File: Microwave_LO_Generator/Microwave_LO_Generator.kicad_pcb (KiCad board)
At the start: 4 copper layers, 53.3 x 42.9 mm, 65 parts, among them J1 Conn_01x02_Male, J2 Conn_01x02_Male, J3 Conn_01x01_Female, J4 Conn_01x05_Male, J5 Conn_01x01_Female, U1 ADF4150HV, U2 LT1962-3.3, U3 LT3010, U4 SMT_24_ADI, U5 LT1962-5, U6 LT1962-5, X1 IQXT-220-1

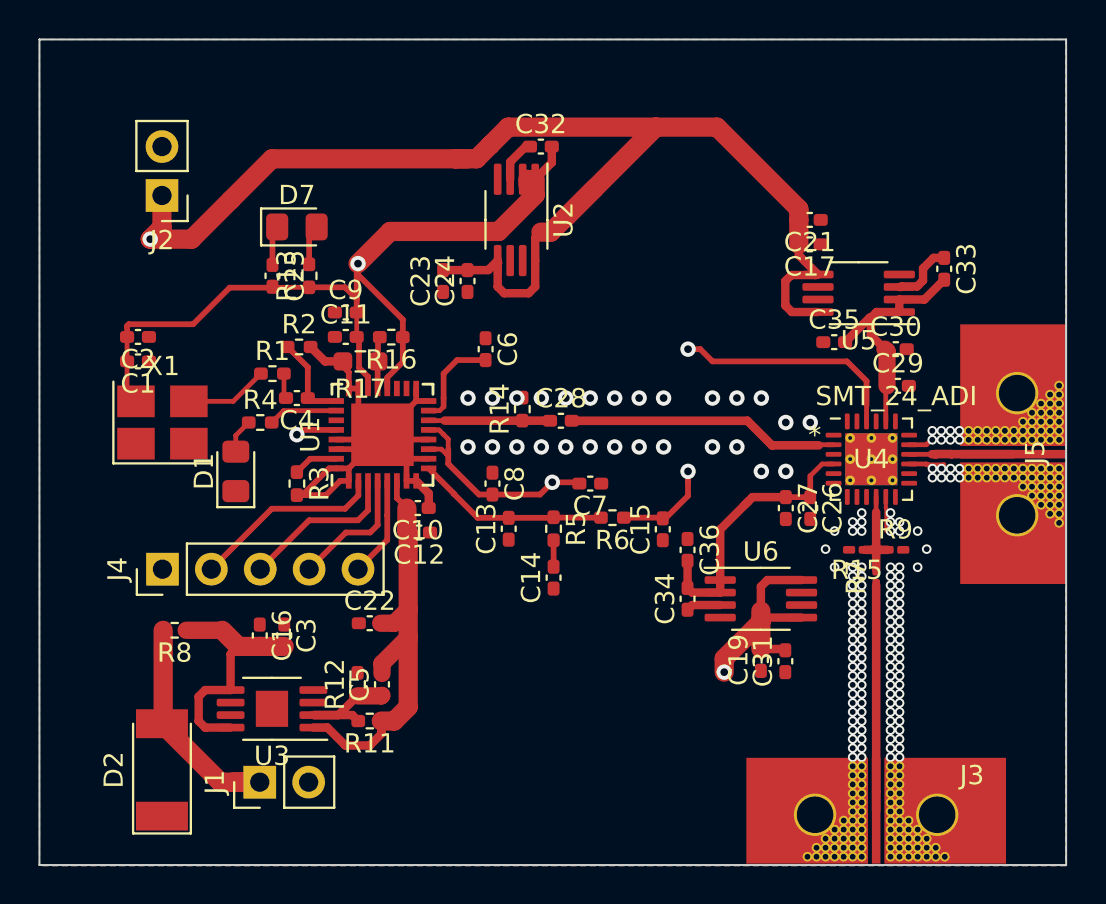
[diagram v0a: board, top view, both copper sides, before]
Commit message: A lot of change
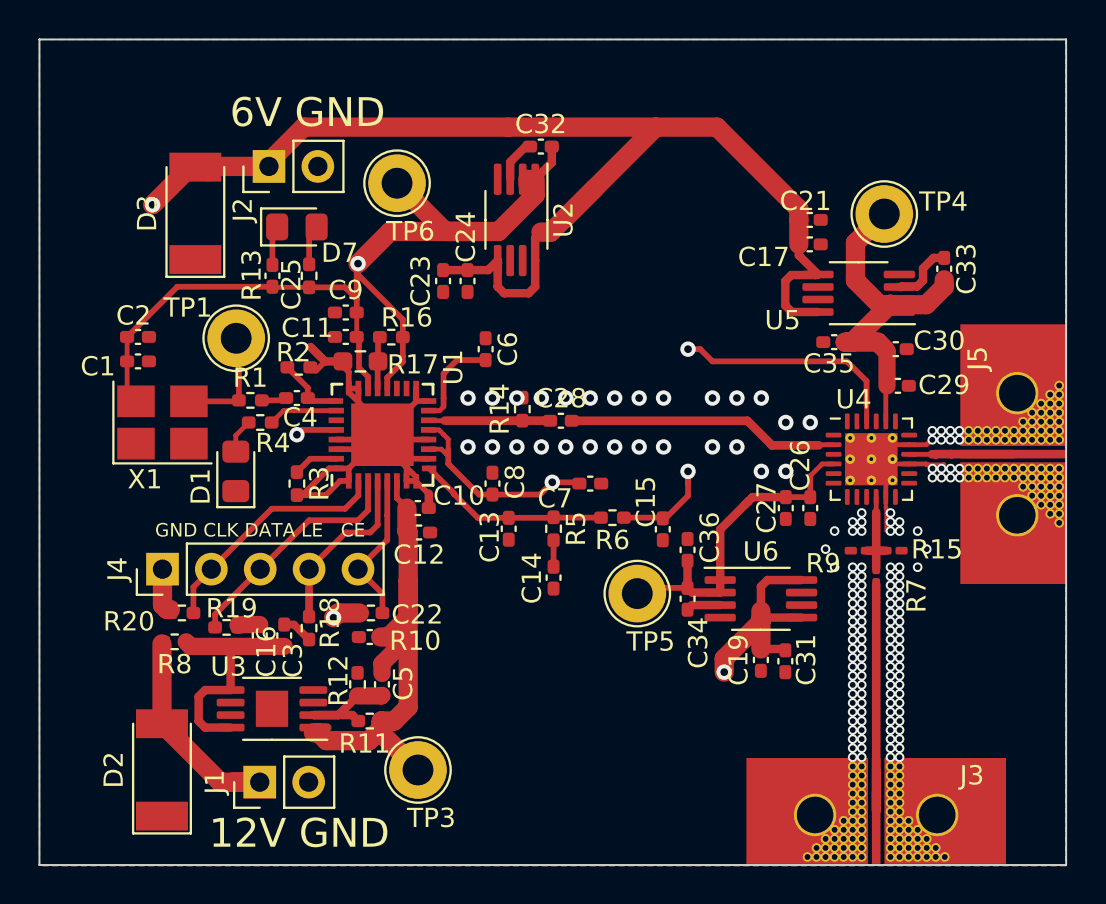
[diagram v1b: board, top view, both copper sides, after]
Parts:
- added D3: DIODE, Diode_SMD:D_MELF, F.Cu at (98.6, 87.4)
- added R10: 10k, Resistor_SMD:R_0402_1005Metric_Pad0.72x0.64mm_HandSolder, F.Cu at (107.7, 108.2)
- added R18: 10k, Resistor_SMD:R_0402_1005Metric_Pad0.72x0.64mm_HandSolder, F.Cu at (104.5, 109.0)
- added R19: 10k, Resistor_SMD:R_0402_1005Metric_Pad0.72x0.64mm_HandSolder, F.Cu at (100.2, 109.0)
- added R20: 10k, Resistor_SMD:R_0402_1005Metric_Pad0.72x0.64mm_HandSolder, F.Cu at (97.9, 108.2)
- added TP1: TestPoint, TestPoint:TestPoint_Loop_D2.60mm_Drill1.6mm_Beaded, F.Cu at (100.7, 93.9)
- added TP3: TestPoint, TestPoint:TestPoint_Loop_D2.60mm_Drill1.6mm_Beaded, F.Cu at (110.2, 116.4)
- added TP4: TestPoint, TestPoint:TestPoint_Loop_D2.60mm_Drill1.6mm_Beaded, F.Cu at (134.4, 87.5)
- added TP5: TestPoint, TestPoint:TestPoint_Loop_D2.60mm_Drill1.6mm_Beaded, F.Cu at (121.6, 107.2)
- added TP6: TestPoint, TestPoint:TestPoint_Loop_D2.60mm_Drill1.6mm_Beaded, F.Cu at (109.1, 85.9)
- J3, J5: value Conn_01x01_Female -> Conn_01x02_Female
- R15, R7, R9: footprint Resistor_SMD:R_0201_0603Metric_Pad0.64x0.40mm_HandSolder -> Microwave_LO_Generator:R_0201_0603_HandSolder_mod
- U1: footprint Package_CSP:LFCSP-32-1EP_5x5mm_P0.5mm_EP3.25x3.25mm -> Microwave_LO_Generator:LFCSP-32-1EP_5x5mm_P0.5mm_mod
- U4: value SMT_24_ADI -> HMC739LP4E; footprint Package_DFN_QFN:QFN-24-1EP_4x4mm_P0.5mm_EP2.7x2.7mm_ThermalVias -> Microwave_LO_Generator:QFN-24-1EP_4x4mm_P0.5mm_EP2.7x2.7mm_ThermalVias_mod
- moved J2 5.76 mm to (102.4, 85.0), turned to 90 degrees
- moved R9 1.90 mm to (133.1, 105.0), turned to 180 degrees
- moved R15 1.90 mm to (134.9, 105.0), turned to 0 degrees
- moved R1 1.80 mm to (101.5, 97.2)
- moved R2 1.06 mm to (104.0, 95.4)
- moved C22 0.72 mm to (107.7, 109.5)
- moved R8 0.60 mm to (97.5, 109.7)
- moved R7 0.06 mm to (134.0, 106.3)
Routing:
- net +3V3: track 88.1 -> 109.1 mm, vias 3 -> 4
- net 0: track 41.8 -> 61.3 mm
- net +5VA: track 12.6 -> 19.3 mm
- net +9V: track 22.7 -> 29.0 mm
- net Net-(J4-Pad3): track 8.39 -> 12.4 mm
- net Net-(J4-Pad5): track 5.21 -> 8.85 mm
- net Net-(J3-Pad1): track 11.7 -> 14.9 mm
- net +6V: track 140.0 -> 137.0 mm
- net +5VD: track 14.7 -> 17.5 mm
- net Net-(J4-Pad4): track 6.80 -> 9.27 mm
- net Net-(J4-Pad2): track 9.98 -> 12.4 mm
- net Net-(R1-Pad1): track 4.34 -> 5.97 mm
- net Net-(C4-Pad1): track 4.78 -> 3.70 mm
- net +12V: track 12.6 -> 12.0 mm
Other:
- net class GND: trace_width 0.2 -> 0.3
- board text added: "12V GND"
- board text added: "6V GND"
- board text added: "GND CLK DATA LE CE"
